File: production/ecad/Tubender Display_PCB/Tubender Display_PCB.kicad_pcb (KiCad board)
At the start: 2 copper layers, 32.5 x 34.5 mm, 2 parts, among them J1 4-1734592-0, J2 4-1734592-0

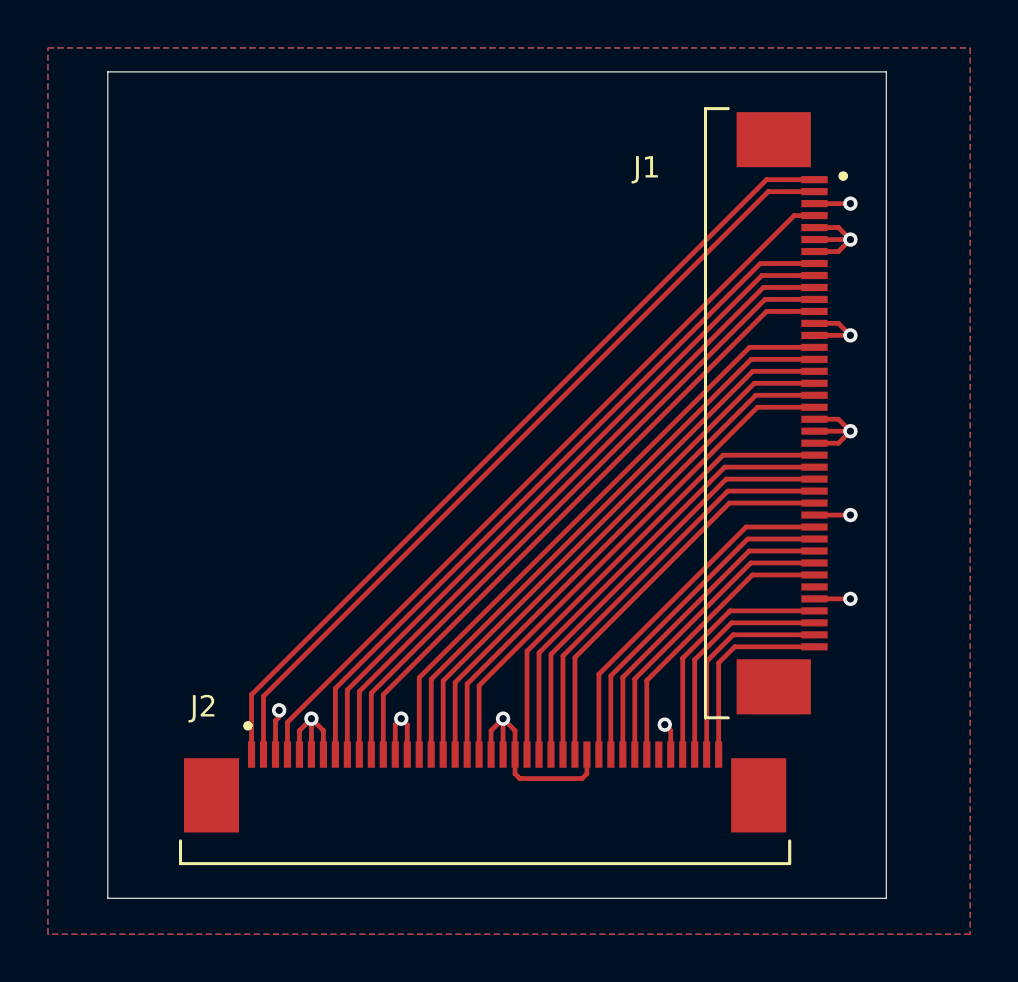
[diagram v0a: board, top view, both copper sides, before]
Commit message: Revert "okay"
This reverts commit a5d04aacf17b2a0e1fddfefa2daa114170fce467, reversing
changes made to 85b8c41c143529192f5821f916a37eef7153b122.
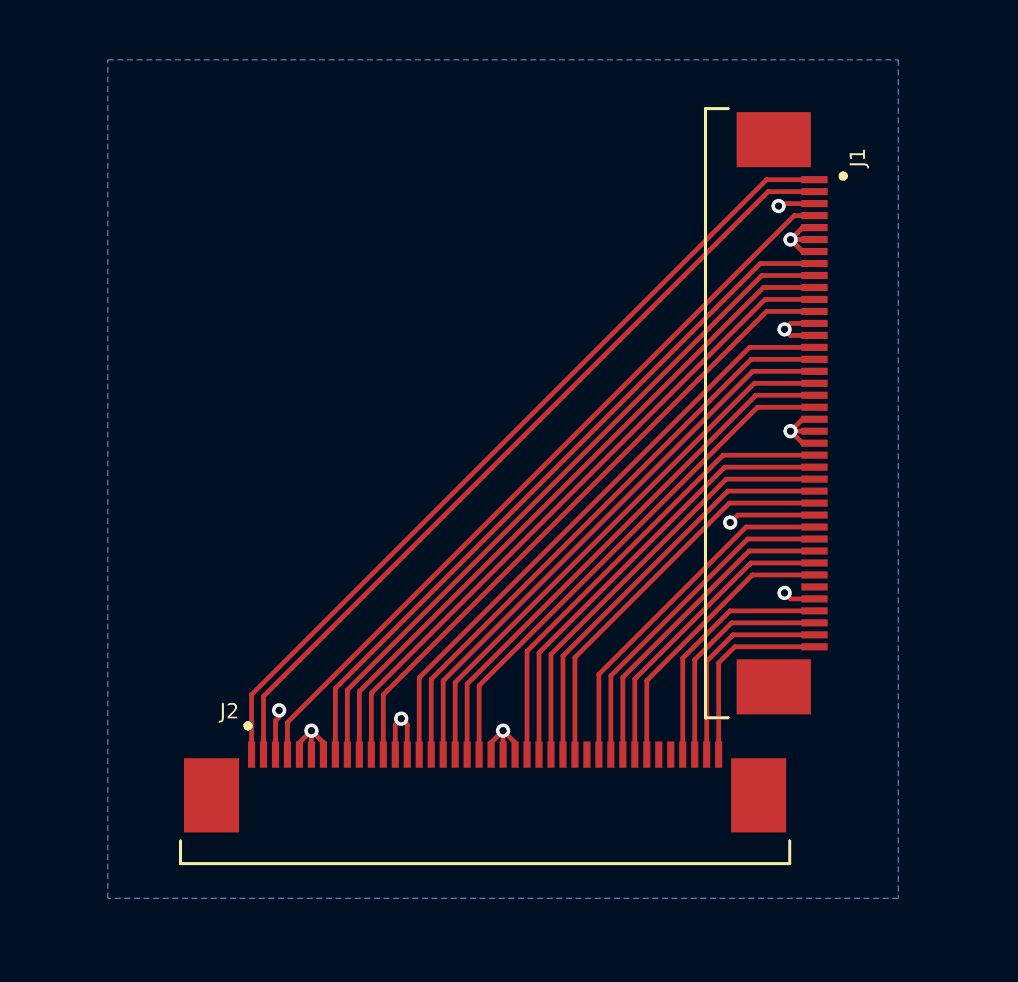
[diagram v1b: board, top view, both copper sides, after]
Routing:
- net GND: track 38.6 -> 28.0 mm, vias 11 -> 10
- removed copper zone on F.Cu, net GND
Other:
- board outline removed
